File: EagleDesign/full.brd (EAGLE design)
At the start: 55 x 55.1 mm, 19 parts, among them IC1 ATMEGA328-28P, T1 2N3904

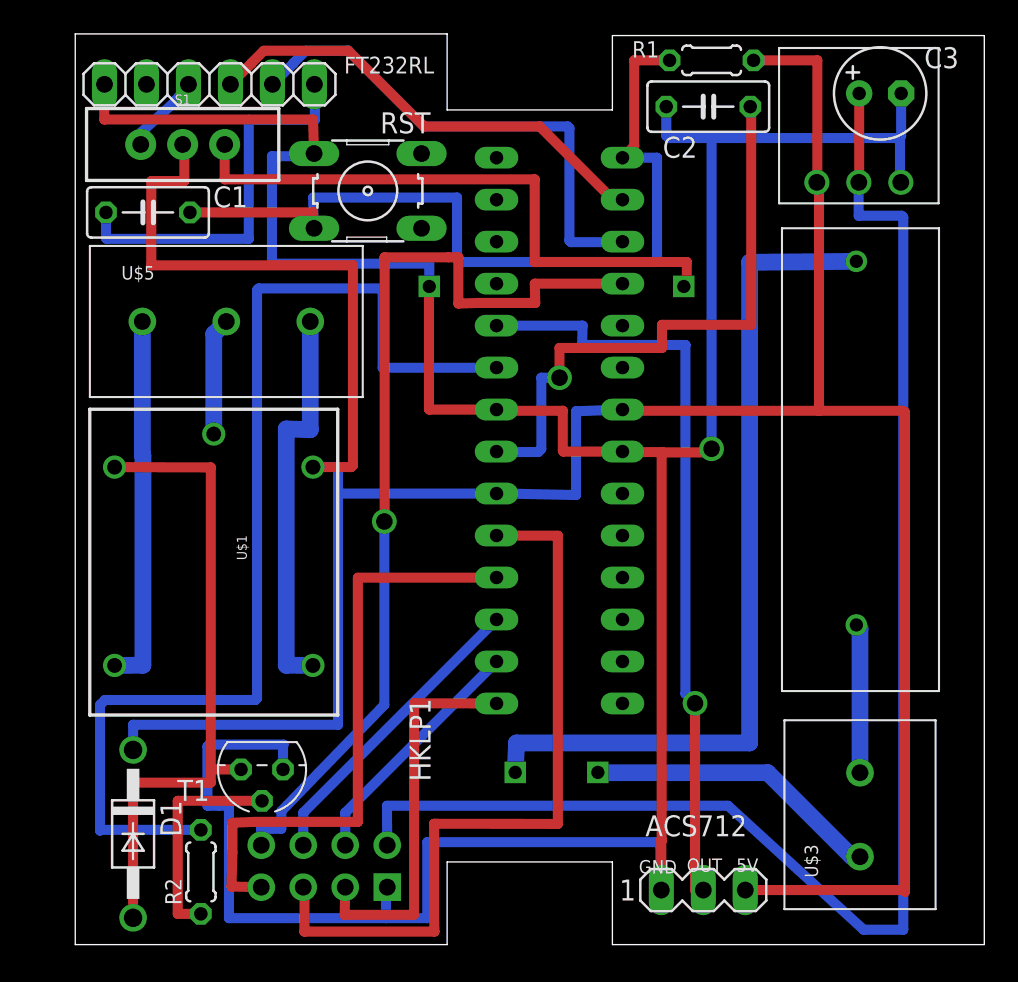
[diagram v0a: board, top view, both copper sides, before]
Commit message: upload V2 of design
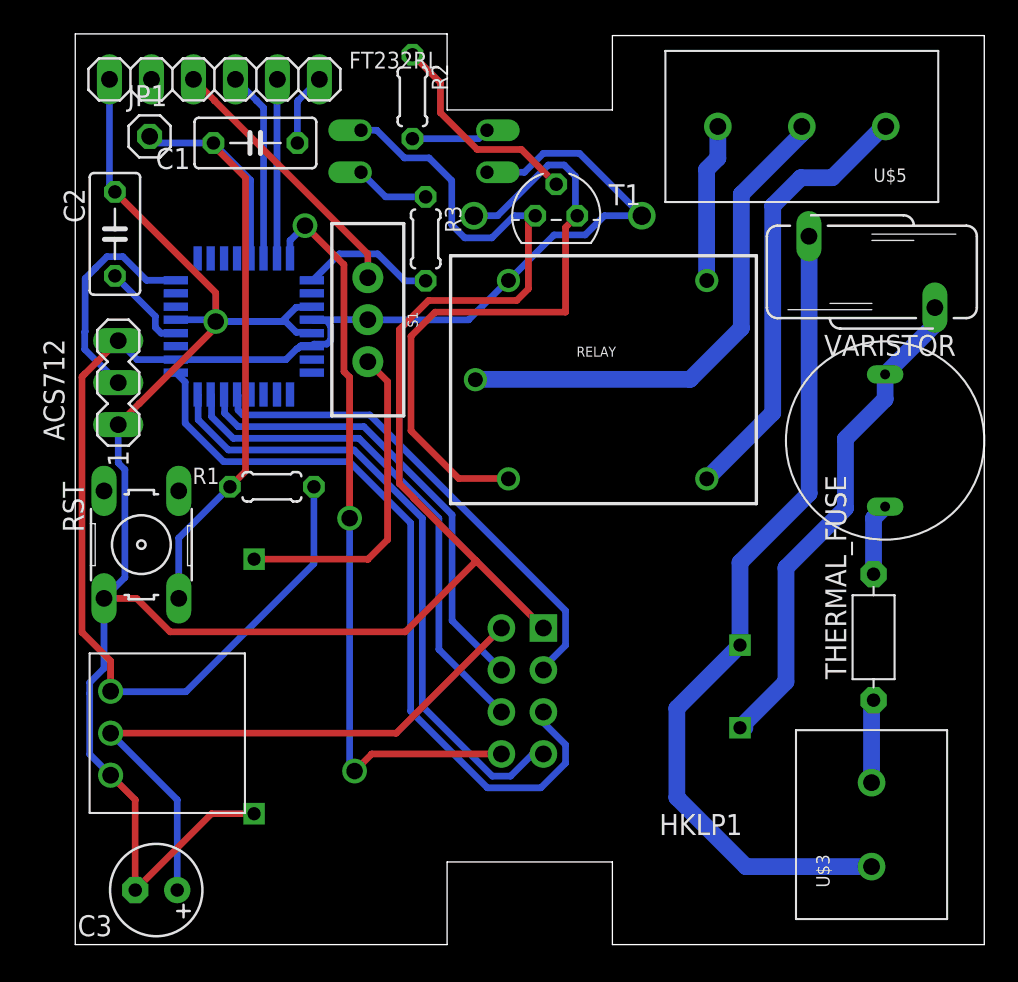
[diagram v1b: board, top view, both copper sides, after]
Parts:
- removed IC1: ATMEGA328-28P, atmega328:DIL28-3
- removed U$1: RELAYPTH, SRD-05VDC-SL-C:SRD-05VDC-SL-C
- removed U$2: (no value), TD-MySensors:AMS1117_VERT
- added 5V->3.3V: (no value), TD-MySensors:AMS1117_VERT
- added ATMEGA328P-AU: ATMEGA328P-AU, Atmel_By_element14_Batch_1-00:QFP80P900X900X120-32N
- added JP1: (no value), pinhead:1X01
- added OPTOCOUPLER: PC817, optocoupler:DIL04
- added R3: 220uK, rcl:0204/5
- added RELAY: SRD-05VDC, SRD-05VDC-SL-C:SRD-05VDC-SL-C
- added THERMAL_FUSE: SF70E, discrete:R-7,5
- added VARISTOR: 10D391K, varistor:S10K385
- FUSE: value BLX-A -> R3-24; device mylib:BLX-A -> mylib:R3-24
- moved C3 65.1 mm to (4.90, 3.30), turned to 180 degrees
- moved R2 48.6 mm to (20.4, 51.3), turned to 270 degrees
- moved ACS712 46.9 mm to (2.60, 34.0), turned to 90 degrees
- moved D1 45.4 mm to (29.2, 44.1), flipped to the bottom, turned to 0 degrees
- moved U$5 41.6 mm to (46.5, 49.5), turned to 180 degrees
- moved T1 37.9 mm to (29.1, 44.1), turned to 0 degrees
- moved R1 37.1 mm to (11.9, 27.7)
- moved C2 36.7 mm to (2.40, 43.0), turned to 270 degrees
- moved RST 25.4 mm to (4.00, 24.2), turned to 90 degrees
- moved S1 15.4 mm to (17.7, 37.8), turned to 180 degrees
- moved FUSE 12.3 mm to (49.0, 30.5)
- moved HKLP1 10.2 mm to (25.5, 15.6), turned to 180 degrees
- moved C1 7.74 mm to (10.9, 48.5), turned to 180 degrees
- moved NRF24L01+ 3.74 mm to (16.3, 13.4), turned to 270 degrees
- moved U$3 0.92 mm to (48.2, 7.26)
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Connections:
- removed net A0: IC1.23, R2.2
- removed net FUSE_C: FUSE.P$2, U$3.P$2
- new net D3: ATMEGA328P-AU.1, R3.2
- new net FU_IN: FUSE.AC_2, THERMAL_FUSE.2
- new net OPTO_IN: OPTOCOUPLER.1, R3.1
- new net RIN: OPTOCOUPLER.3, R2.2
- new net TR_IN: THERMAL_FUSE.1, U$3.P$2
- net +3V3: now also 5V->3.3V.3V3; no longer U$2.3V3
- net +5V: now also 5V->3.3V.5V, ATMEGA328P-AU.18, ATMEGA328P-AU.4, ATMEGA328P-AU.6, OPTOCOUPLER.4, RELAY.COIL1; no longer IC1.20, IC1.7, U$1.COIL1, U$2.5V
- net A1: now also ATMEGA328P-AU.24; no longer IC1.24
- net AC1_F: now also FUSE.AC_1, VARISTOR.1; no longer FUSE.P$1
- net AC2: now also VARISTOR.2
- net AREF: now also ATMEGA328P-AU.20; no longer IC1.21
- net D10: now also ATMEGA328P-AU.14; no longer IC1.16
- net D2: now also ATMEGA328P-AU.32; no longer IC1.4
- net D9: now also ATMEGA328P-AU.13; no longer IC1.15
- net GND: now also 5V->3.3V.GND, ATMEGA328P-AU.21, ATMEGA328P-AU.3, ATMEGA328P-AU.5, OPTOCOUPLER.2; no longer IC1.22, IC1.8, U$2.GND
- net MISO: now also ATMEGA328P-AU.16; no longer IC1.18
- net MOSI: now also ATMEGA328P-AU.15; no longer IC1.17
- net RST: now also ATMEGA328P-AU.29, JP1.1; no longer IC1.1
- net RX: now also ATMEGA328P-AU.31; no longer IC1.3
- net R_CENTER: now also RELAY.SWCOMMON; no longer U$1.SWCOMMON
- net R_IN: now also RELAY.COIL0; no longer U$1.COIL0
- net R_LEFT: now also RELAY.SWOPEN; no longer U$1.SWOPEN
- net R_RIGHT: now also RELAY.SWCLOSED; no longer U$1.SWCLOSED
- net SCK: now also ATMEGA328P-AU.17; no longer IC1.19
- net TX: now also ATMEGA328P-AU.30; no longer IC1.2
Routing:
- net +5V: track 170.5 -> 92.7 mm
- net A0: track 67.4 -> 0.00 mm
- net +3V3: track 89.8 -> 37.4 mm
- net AC2: track 18.0 -> 50.8 mm
- net A1: track 46.4 -> 13.8 mm, vias 1 -> 0
- net AREF: track 36.3 -> 5.51 mm, vias 1 -> 0
- net GND: track 184.0 -> 155.7 mm
- net R_CENTER: track 7.12 -> 31.1 mm
- net AC1_F: track 51.4 -> 30.6 mm
- net RX: track 30.8 -> 10.8 mm
- net DTR: track 23.6 -> 4.40 mm
- net PSU_VIN: track 36.6 -> 19.9 mm
- net TX: track 28.3 -> 11.5 mm
- net R_LEFT: track 23.9 -> 9.61 mm
- net D10: track 14.9 -> 28.1 mm
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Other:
- board text removed: "5V"
- board text removed: "GND"
- board text removed: "OUT"
